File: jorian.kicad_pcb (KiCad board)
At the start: 2 copper layers, 98.9 x 100 mm, 97 parts, among them J1 MicroUSB, J2 USB-C, J3 MicroUSB, J4 USB-C, J5 MJ-4PP-9, J6 lipo_charger, J7 lipo_header, SW1 SW_SPDT, U3 LP3990-3.3v

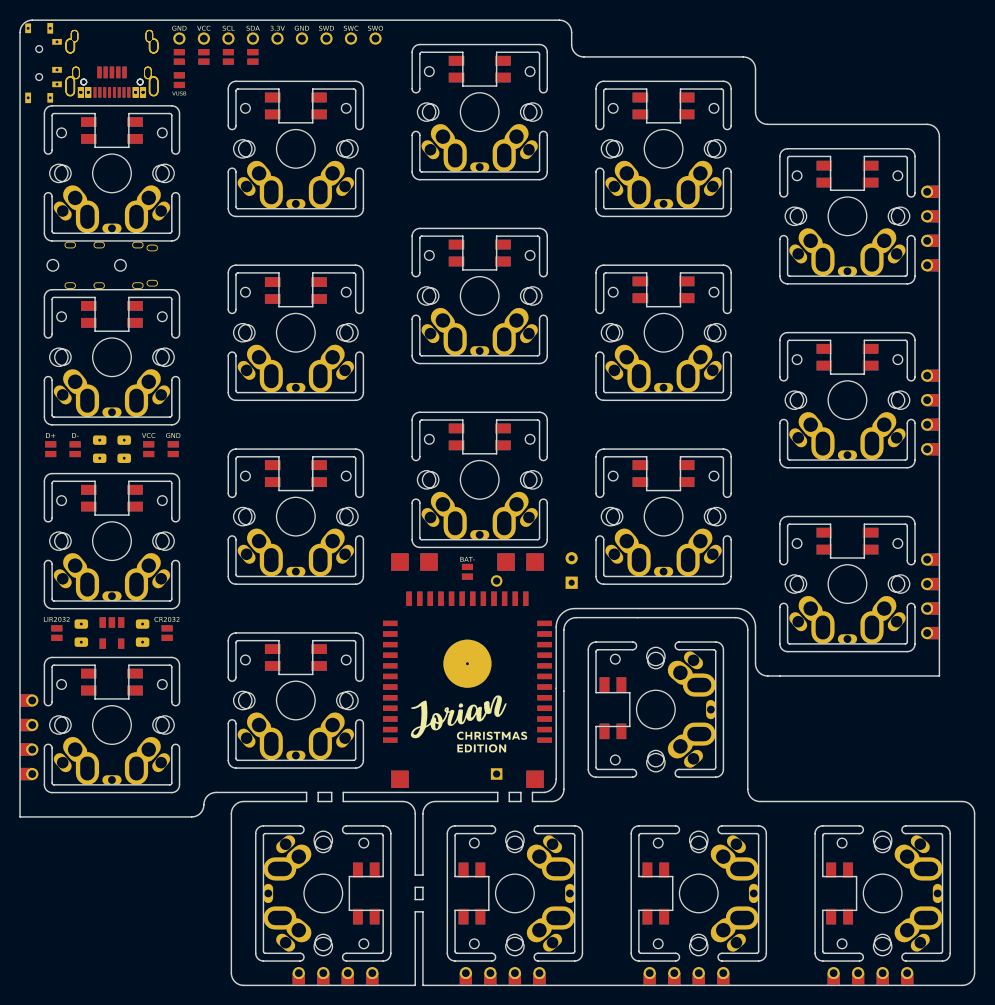
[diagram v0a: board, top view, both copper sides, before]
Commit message: sent files
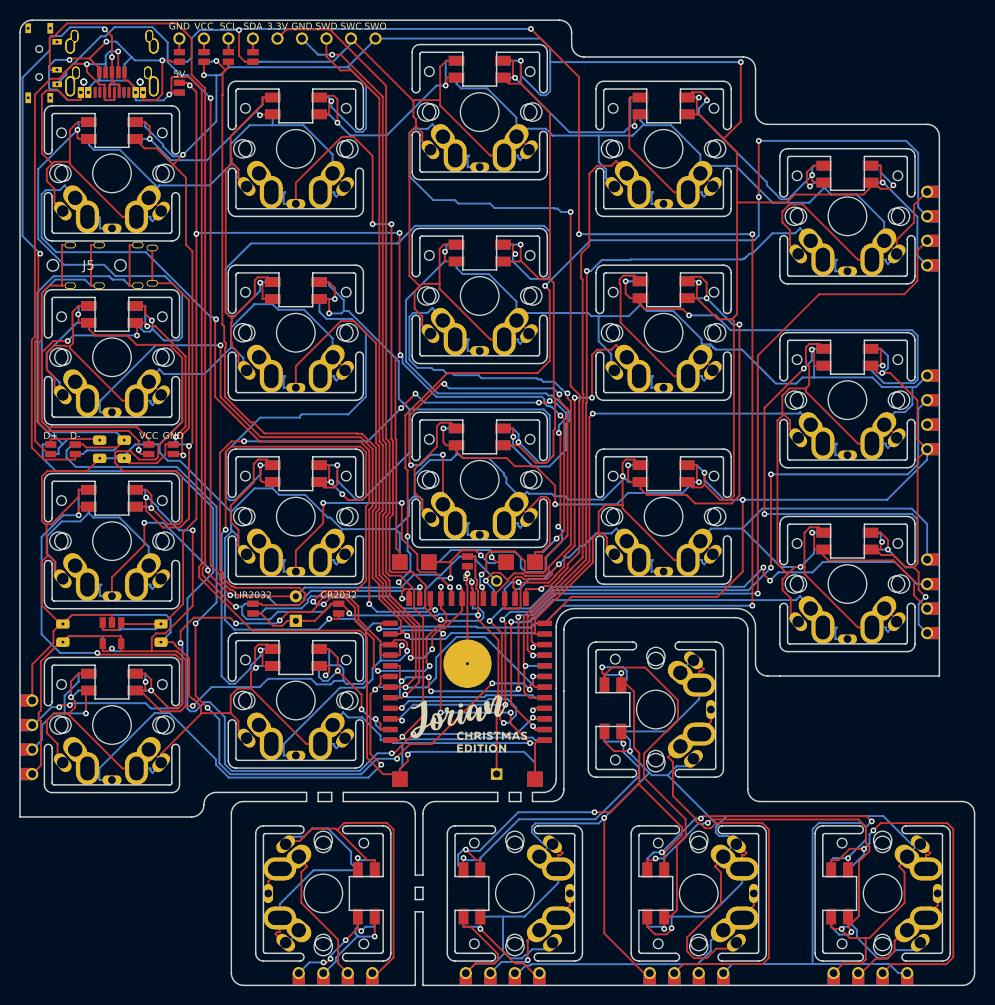
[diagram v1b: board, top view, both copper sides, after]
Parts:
- C1, C2: value 1nF -> 1uF
- J7: value lipo_header -> Conn_01x02
- JP1: value BAT+ -> B+
- JP10: value BAT- -> B-
- JP15, JP17: value VUSB -> 5V
- moved J7 28.8 mm to (69.8, 99.7)
- moved JP18 20.5 mm to (65.4, 99.7)
- moved JP19 20.5 mm to (65.4, 99.7)
- moved JP20 18.0 mm to (74.3, 99.7)
- moved JP21 18.0 mm to (74.3, 99.7)
- moved C1 8.26 mm to (55.9, 102.2)
- moved C2 8.26 mm to (45.7, 102.2)
- moved JP1 1.08 mm to (87.6, 94.8)
- moved JP10 1.08 mm to (87.6, 94.8)
- moved JP15 0.77 mm to (57.8, 45.7), turned to 180 degrees
- moved JP17 0.77 mm to (57.8, 45.7), turned to 0 degrees
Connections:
- net /SWC renamed SWC
- net /SWD renamed SWD
- J6 pad 6: OUT- -> GND
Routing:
- net GND: track 0.00 -> 1118.3 mm, vias 0 -> 13
- net VCC: track 0.00 -> 656.5 mm, vias 0 -> 27
- net /GND_B: track 0.00 -> 225.2 mm, vias 0 -> 4
- net OUT+: track 0.00 -> 167.9 mm, vias 0 -> 6
- net SDA: track 0.00 -> 164.6 mm, vias 0 -> 6
- net /VCC_B: track 0.00 -> 132.2 mm, vias 0 -> 7
- net VUSB: track 0.00 -> 127.6 mm, vias 0 -> 2
- net /S1: track 0.00 -> 112.2 mm, vias 0 -> 6
- net /S19: track 0.00 -> 106.9 mm, vias 0 -> 6
- net Net-(BT1-Pad1): track 0.00 -> 105.5 mm, vias 0 -> 1
- net /S20: track 0.00 -> 102.7 mm, vias 0 -> 6
- net LIPO-: track 0.00 -> 102.1 mm, vias 0 -> 8
- net SWO: track 0.00 -> 101.5 mm, vias 0 -> 1
- net BAT+: track 0.00 -> 94.8 mm, vias 0 -> 1
- net SWD: track 0.00 -> 94.0 mm, vias 0 -> 1
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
